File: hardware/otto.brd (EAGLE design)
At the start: 56 x 48.5 mm, 79 parts, among them U1 BLU, U2 TPS61230DRCR, U3 PAM8302AASCR, U4 BMX160, U5 TPS2115AIPWRQ1-SON8, U6 MIC-PDM-MP23DB01HPTR

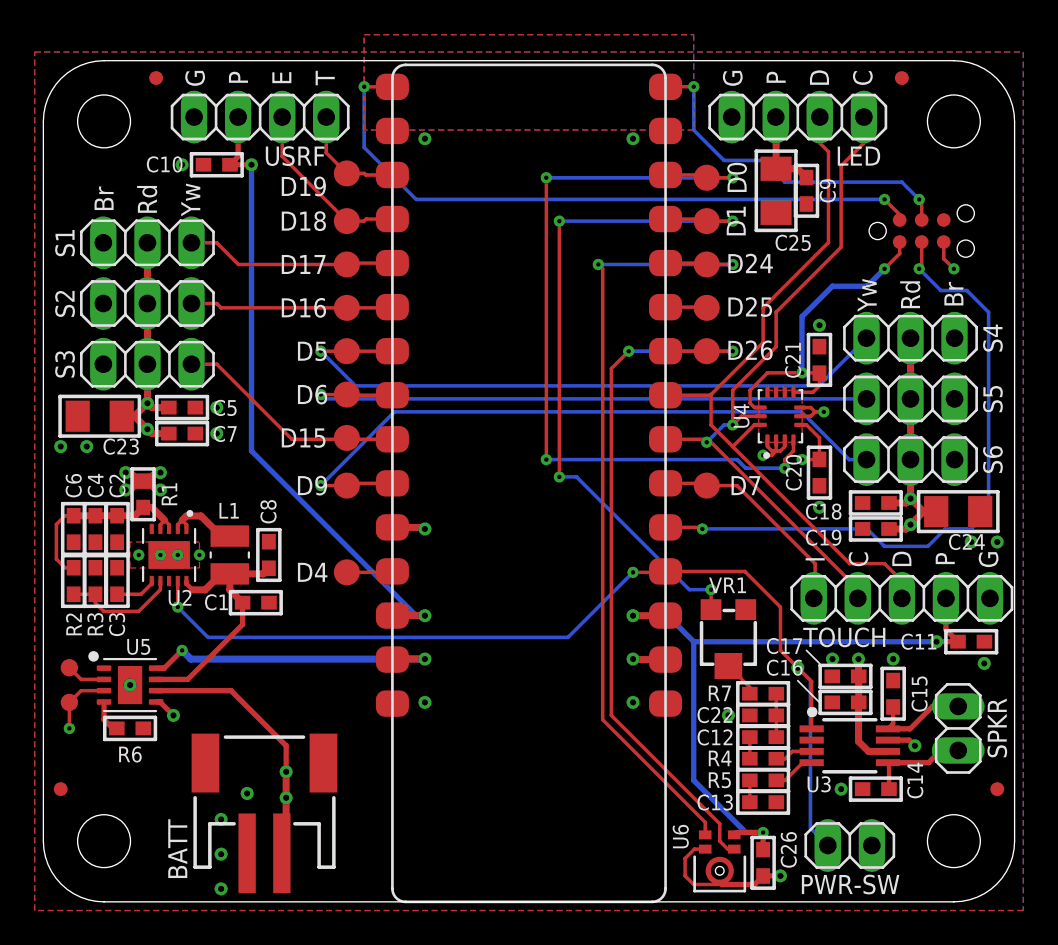
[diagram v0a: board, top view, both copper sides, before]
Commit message: Lots of PCB changes v2 (see hardware readme)
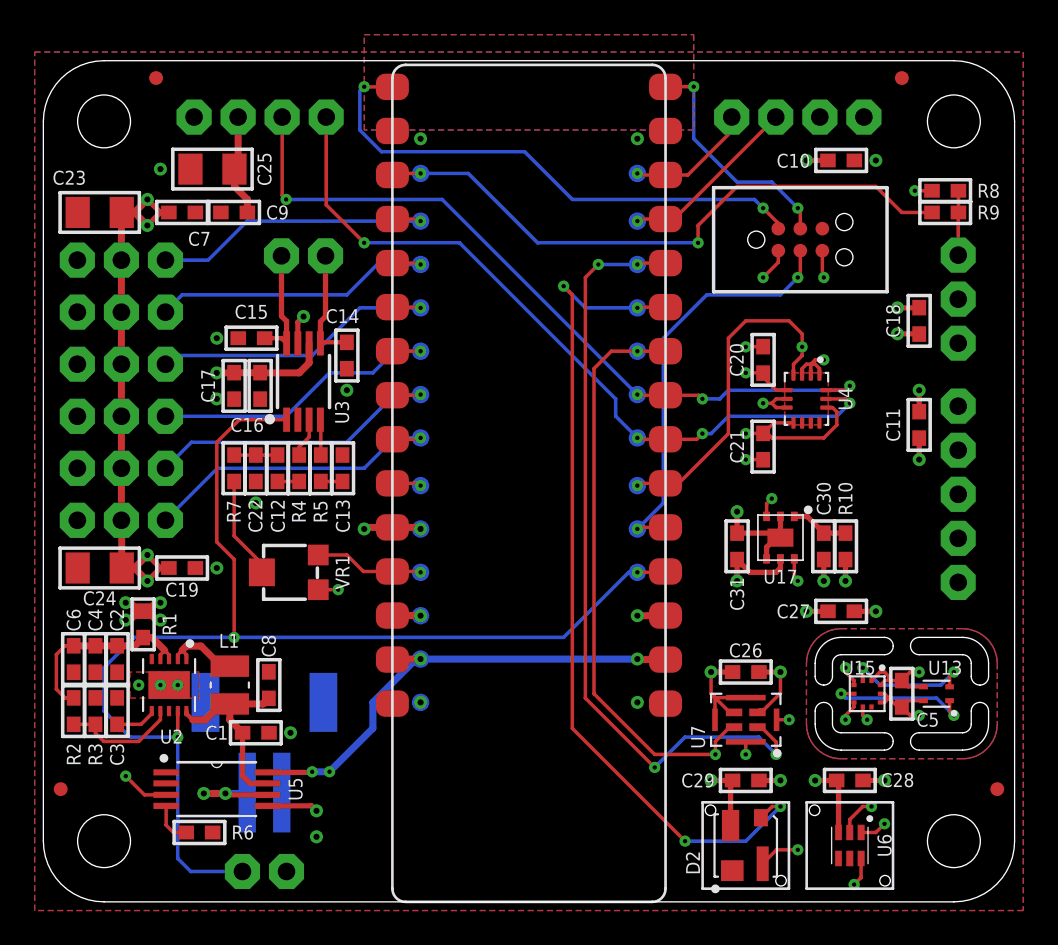
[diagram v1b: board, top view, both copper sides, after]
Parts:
- removed D3: TPSQTP10R, otto:TP10R
- added 3V3, GND, PEN, RST, SCL, SDA, VBS, VBT: TPSQTP10R, otto:TP10R
- added C27, C28, C29: 100n, otto:_0603
- added C30, C31: 10u, otto:_0603
- added H1, H2: (no value), otto:VLP-XXX-X
- added PIR: (no value), otto:1X03
- added R10: 4.7, otto:_0603
- added R8, R9: 100k, otto:_0603
- added U13: SHT4X, otto:SHT4X-DFN4
- added U15: LPS22HB, otto:HLGA-10L
- added U17: SGP41, otto:SGP41
- added U7: SPK0641HT4H, otto:SPK0641HT4H-1
- C18, C5: value 10u -> 100n
- D0, D1, D15, D16, D17, D18, D19, D24, D25, D26, D4, D5, D6, D7, D9: value TPSQTP15R -> TPSQTP10R; device otto:TP15R -> otto:TP10R
- D2: value TPSQTP10R -> SK6812MINI; device otto:TP10R -> otto:SK6812MINI
- U5: value TPS2115AIPWRQ1-SON8 -> TPS2115AIPWRQ1; device otto:SON65P300X300X100-9N -> otto:SOP65P640X120-8N
- U6: value MIC-PDM-MP23DB01HPTR -> APDS-9250; device otto:MP23DB01HPTR -> otto:SON65P200X200X75-6N
- moved C24 49.6 mm to (3.25, 19.2), turned to 0 degrees
- moved SPKR 46.6 mm to (15.0, 37.2), flipped to the bottom, turned to 0 degrees
- moved S4 45.7 mm to (4.50, 28.0), flipped to the bottom
- moved S5 45.7 mm to (4.50, 25.0), flipped to the bottom
- moved S6 45.6 mm to (4.50, 22.0), flipped to the bottom
- moved C5 44.7 mm to (49.5, 12.0), turned to 270 degrees
- moved C15 42.3 mm to (12.0, 32.5), turned to 0 degrees
- moved D2 40.3 mm to (40.5, 3.25), turned to 90 degrees
- moved C19 40.1 mm to (8.00, 19.2), turned to 180 degrees
- moved C14 39.4 mm to (17.5, 31.5), turned to 90 degrees
- moved C17 39.0 mm to (11.0, 29.8), turned to 270 degrees
- moved C16 38.4 mm to (12.5, 29.8), turned to 270 degrees
- moved U3 37.9 mm to (15.0, 30.0), turned to 0 degrees
- moved C10 36.0 mm to (46.0, 42.8), turned to 180 degrees
- moved PWR-SW 33.8 mm to (12.8, 1.75), flipped to the bottom, turned to 0 degrees
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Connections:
- removed net D0/IMU_INT: D0.TP, U1.13, U4.4
- removed net D1/SPKR: D1.TP, U1.12, VR1.3
- removed net D15/SM3: D15.TP, S3.3, U1.24
- removed net D16/SM2: D16.TP, S2.3, U1.21
- removed net D17/SM1: D17.TP, S1.3, U1.20
- removed net D18/USRF_ECHO: D18.TP, U1.19, USRF.3
- removed net D19/USRF_TRIG: D19.TP, U1.18, USRF.4
- removed net D25/MOSI: D25.TP, U1.10
- removed net D4: D4.TP, U1.27
- removed net D7/TOUCH_INT: D7.TP, TOUCH.5, U1.6
- removed net D9/SM6: D9.TP, S6.3, U1.25
- removed net N$6: D2.TP, U5.2
- new net 3V3_A: C30.1, R10.2, U17.1
- new net D0/USRF_TRIG: D0.TP, U1.13, USRF.4
- new net D1/USRF_ECHO: D1.TP, U1.12, USRF.3
- new net D15/SM6: D15.TP, S6.3, U1.24
- new net D16/SM3: D16.TP, S3.3, U1.21
- new net D17/SM2: D17.TP, S2.3, U1.20
- new net D18/SM1: D18.TP, S1.3, U1.19
- new net D19/PIR: D19.TP, R9.1, U1.18
- new net D25/MOSI/PIX: D2.3, D25.TP, U1.10
- new net D4/SPKR: D4.TP, U1.27, VR1.3
- new net D7/IMU_INT: D7.TP, U1.6, U4.4
- new net D9/TOUCH_INT: D9.TP, TOUCH.5, U1.25
- new net N$5: PIR.3, R8.2, R9.2
- net !RST: now also RST.TP
- net 3V3: now also 3V3.TP, C18.2, C27.1, C28.1, C29.1, C31.1, C5.1, D2.4, PIR.2, R10.1, U13.3, U15.1, U15.10, U15.6, U17.5, U6.3, U7.4; no longer U6.5
- net 5V0: no longer C18.2, C5.2
- net D22/SDA: now also SDA.TP, U13.1, U15.4, U17.3, U6.2
- net D23/SCL: now also SCL.TP, U13.2, U15.2, U17.6, U6.1
- net D24/MISO/MDAT: now also U7.1; no longer U6.1
- net D26/SCLK/MCLK: now also U7.2; no longer U6.4
- net GND: now also C27.2, C28.2, C29.2, C30.2, C31.2, C5.2, D2.2, GND.TP, PIR.1, R8.1, U13.4, U15.3, U15.5, U15.8, U15.9, U17.2, U17.4, U17.EP, U6.6, U7.3, U7.5, U7.6, U7.7, U7.8; no longer C5.1, D3.TP, U5.9, U6.2, U6.3
- net PWR_EN: now also PEN.TP
- net VBAT: now also VBT.TP
- net VBUS: now also VBS.TP
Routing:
- net 3V3: track 132.2 -> 68.6 mm, vias 8 -> 16
- net D25/MOSI/PIX: track 0.00 -> 49.0 mm, vias 0 -> 4
- net D0/IMU_INT: track 46.7 -> 0.00 mm, vias 4 -> 0
- net GND: track 22.8 -> 66.1 mm, vias 34 -> 41
- net D1/SPKR: track 41.3 -> 0.00 mm, vias 4 -> 0
- net D9/SM6: track 38.5 -> 0.00 mm, vias 1 -> 0
- net D19/PIR: track 0.00 -> 35.4 mm, vias 0 -> 2
- net D5/SM4: track 37.6 -> 17.9 mm
- net D7/IMU_INT: track 0.00 -> 19.5 mm, vias 0 -> 2
- net D15/SM6: track 0.00 -> 18.3 mm, vias 0 -> 1
- net D16/SM3: track 0.00 -> 17.7 mm, vias 0 -> 1
- net D6/SM5: track 35.7 -> 18.1 mm
- net D17/SM2: track 0.00 -> 17.5 mm, vias 0 -> 1
- net D18/SM1: track 0.00 -> 17.3 mm, vias 0 -> 1
- net D22/SDA: track 41.3 -> 56.1 mm, vias 0 -> 8
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- added copper zone on layer 15, net 3V3
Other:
- outline, holes or cut-outs redrawn
- board text added: "+"
- board text added: "O++O v2A 2021.12"
- board text removed: "O++O [B] 2021.12"
